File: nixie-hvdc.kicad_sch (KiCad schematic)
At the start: 13 parts, among them Q1 IRF740, U1 MAX1771xSA

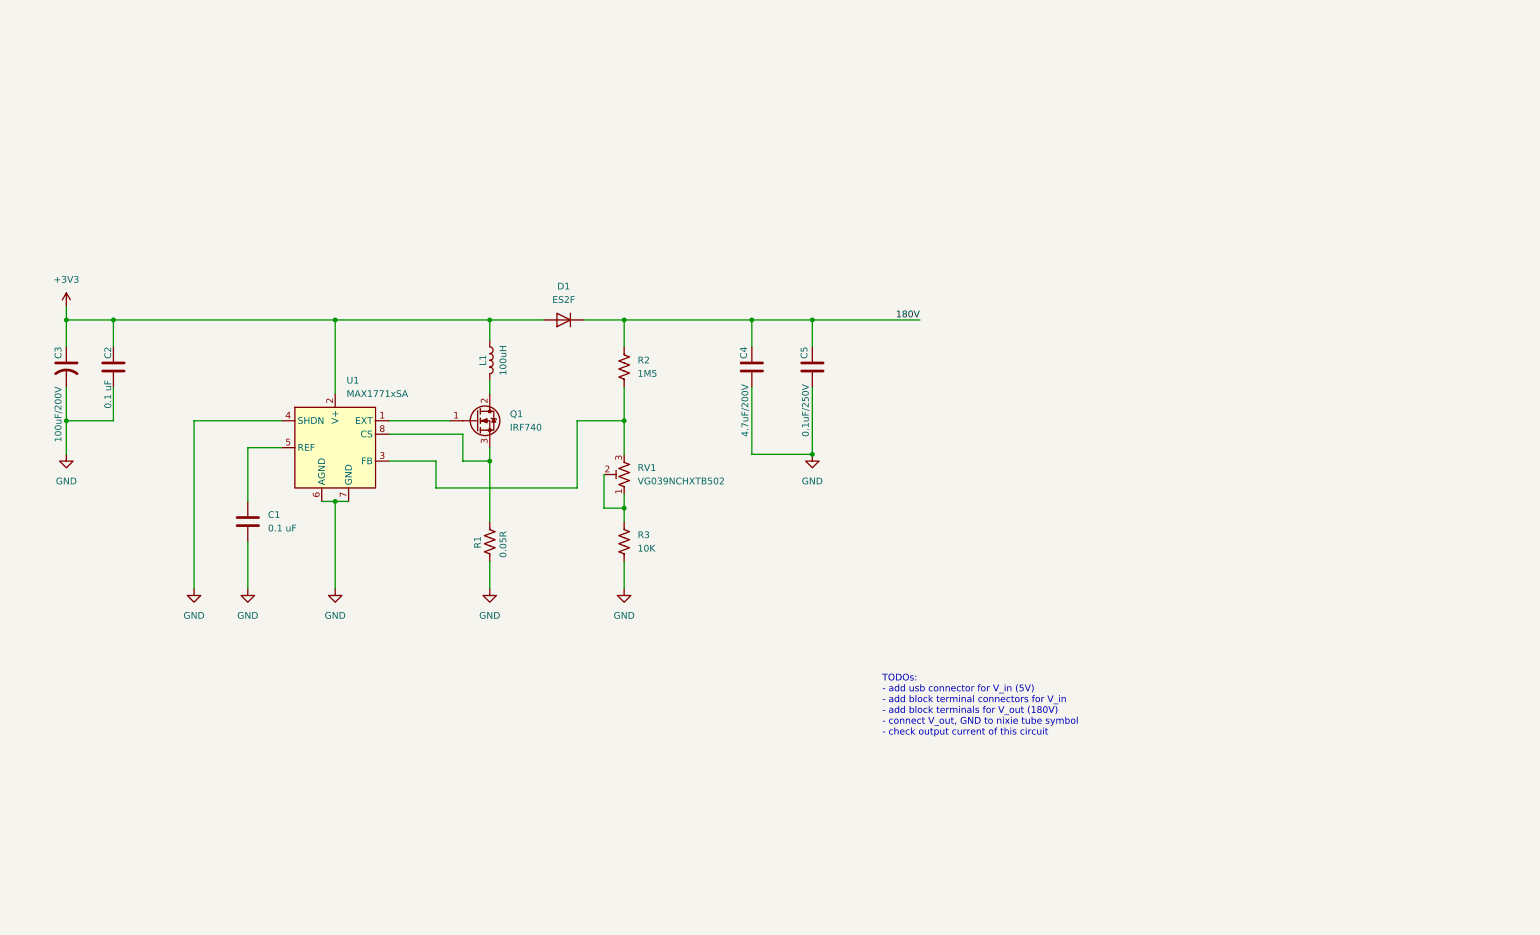
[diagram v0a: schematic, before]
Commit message: almost done
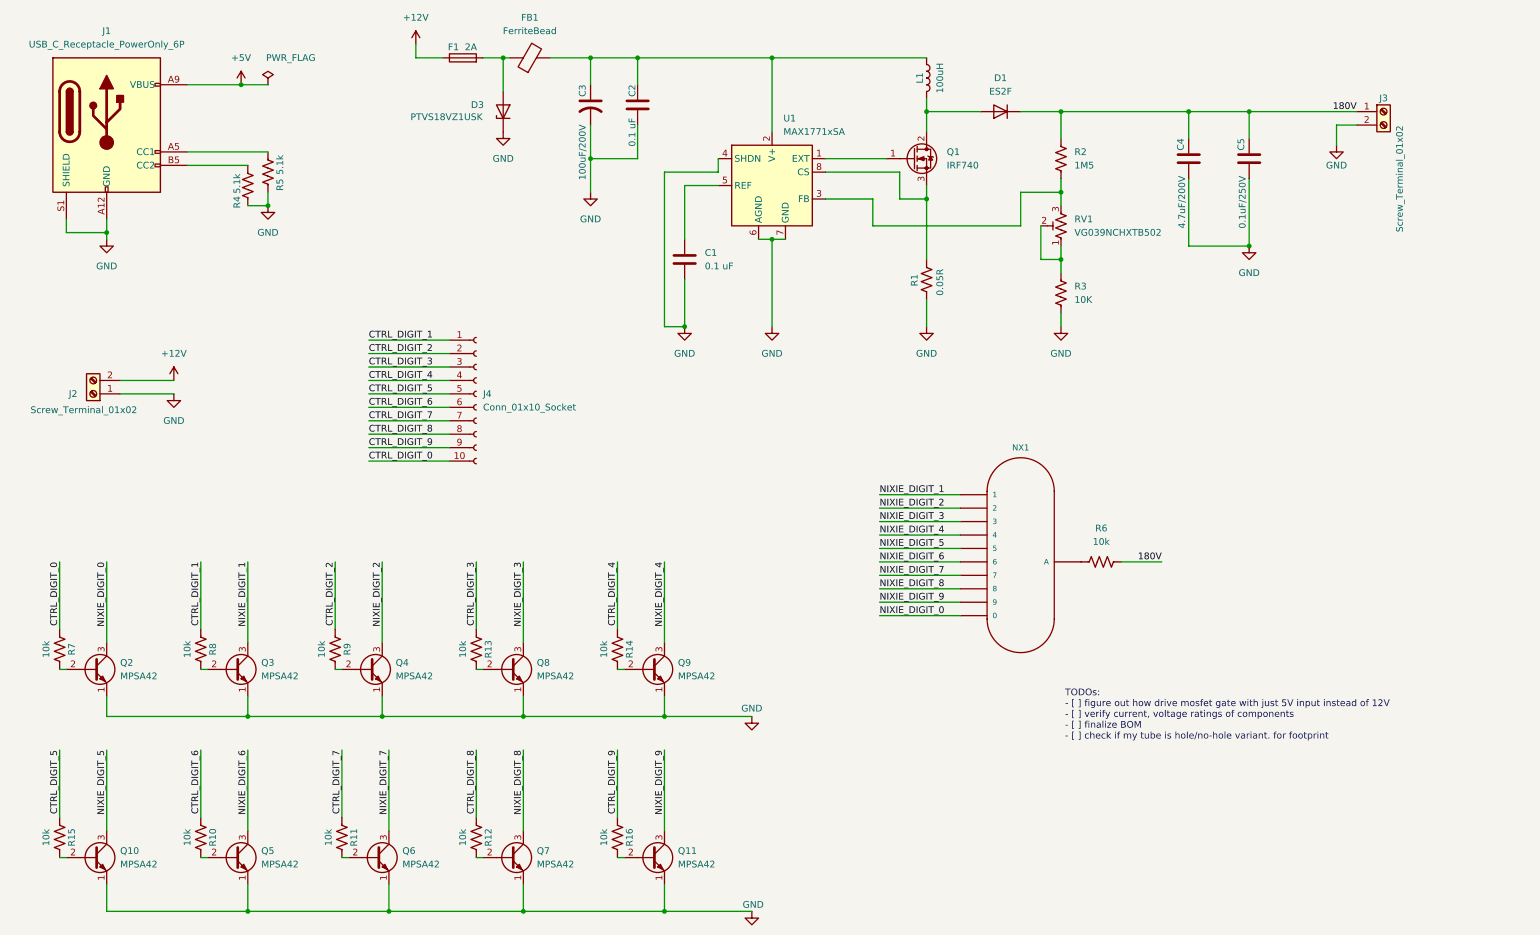
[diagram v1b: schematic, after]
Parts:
- added D3: PTVS18VZ1USK, Diode_SMD:Nexperia_DSN1608-2_1.6x0.8mm, symbol Diode:PTVS18VZ1USK
- added F1: 2A, symbol Device:Fuse
- added FB1: FerriteBead, symbol Device:FerriteBead
- added J1: USB_C_Receptacle_PowerOnly_6P, Connector_USB:USB_C_Receptacle_HRO_TYPE-C-31-M-17, symbol Connector:USB_C_Receptacle_PowerOnly_6P
- added J2, J3: Screw_Terminal_01x02, TerminalBlock_Phoenix:TerminalBlock_Phoenix_MKDS-1,5-2-5.08_1x02_P5.08mm_Horizontal, symbol Connector:Screw_Terminal_01x02
- added J4: Conn_01x10_Socket, Connector_PinHeader_2.54mm:PinHeader_1x10_P2.54mm_Vertical, symbol Connector:Conn_01x10_Socket
- added NX1: IN-12A, nixies-us:nixies-us-IN-12-DSUB-NOHOLE, symbol nixies-us:IN-12A
- added Q10, Q11, Q2, Q3, Q4, Q5, Q6, Q7, Q8, Q9: MPSA42, Package_TO_SOT_THT:TO-92_Inline, symbol Transistor_BJT:MPSA42
- added R10, R11, R12, R13, R14, R15, R16, R6, R7, R8, R9: 10k, symbol Device:R_US
- added R4, R5: 5.1k, symbol Device:R_US
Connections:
- net 180V: now also J3.1 (Pin_1), R6.2
- net GND: now also D3.1 (K), J1.A12 (GND), J1.B12 (GND), J1.S1 (SHIELD), J2.1 (Pin_1), J3.2 (Pin_2), Q10.1 (E), Q11.1 (E), Q2.1 (E), Q3.1 (E), Q4.1 (E), Q5.1 (E), Q6.1 (E), Q7.1 (E), Q8.1 (E), Q9.1 (E), R4.2, R5.2
- net at L1.2, Q1.2 (D): now also D1.2 (A)
- net +3V3: no longer names the net of C2.1, C3.1, L1.1, U1.2 (V+)
- net +3V3: now also FB1.2; no longer D1.2 (A)
- new net: Q2.2 (B), R7.2
- new net: Q6.2 (B), R11.2
- new net: Q10.2 (B), R15.2
- new net: Q8.2 (B), R13.2
- new net: Q11.2 (B), R16.2
- new net: Q3.2 (B), R8.2
- new net: Q5.2 (B), R10.2
- new net: J1.B5 (CC2), R4.1
- new net: Q7.2 (B), R12.2
- new net: NX1.A, R6.1
- new net: J1.A5 (CC1), R5.1
- new net: Q9.2 (B), R14.2
- new net: D3.2 (A), F1.2, FB1.1
- new net: Q4.2 (B), R9.2
- new net +12V: F1.1, J2.2 (Pin_2)
- new net +5V: J1.A9 (VBUS), J1.B9 (VBUS)
- new net CTRL_DIGIT_0: J4.10 (Pin_10), R7.1
- new net CTRL_DIGIT_1: J4.1 (Pin_1), R8.1
- new net CTRL_DIGIT_2: J4.2 (Pin_2), R9.1
- new net CTRL_DIGIT_3: J4.3 (Pin_3), R13.1
- new net CTRL_DIGIT_4: J4.4 (Pin_4), R14.1
- new net CTRL_DIGIT_5: J4.5 (Pin_5), R15.1
- new net CTRL_DIGIT_6: J4.6 (Pin_6), R10.1
- new net CTRL_DIGIT_7: J4.7 (Pin_7), R11.1
- new net CTRL_DIGIT_8: J4.8 (Pin_8), R12.1
- new net CTRL_DIGIT_9: J4.9 (Pin_9), R16.1
- new net NIXIE_DIGIT_0: NX1.0, Q2.3 (C)
- new net NIXIE_DIGIT_1: NX1.1, Q3.3 (C)
- new net NIXIE_DIGIT_2: NX1.2, Q4.3 (C)
- new net NIXIE_DIGIT_3: NX1.3, Q8.3 (C)
- new net NIXIE_DIGIT_4: NX1.4, Q9.3 (C)
- new net NIXIE_DIGIT_5: NX1.5, Q10.3 (C)
- new net NIXIE_DIGIT_6: NX1.6, Q5.3 (C)
- new net NIXIE_DIGIT_7: NX1.7, Q6.3 (C)
- new net NIXIE_DIGIT_8: NX1.8, Q7.3 (C)
- new net NIXIE_DIGIT_9: NX1.9, Q11.3 (C)
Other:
- note added: "TODOs: - [ ] figure out how drive mosfet gate with just 5V input instead of 12V - [ ] verify current, voltage ratings of components - [ ] finalize BOM - [ ] check if my tube is hole/no-hole variant. for footprint"
- note removed: "TODOs: - add usb connector for V_in (5V) - add block terminal connectors for V_in - add block terminals for V_out (180V) - connect V_out, GND to nixie tube symbol - check output current of this circuit"
- moved on the sheet: C1, C2, C3, C4, C5, D1, L1, Q1, R1, R2, R3, RV1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
